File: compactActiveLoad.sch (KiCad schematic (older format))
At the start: 35 parts, among them CON1 Keystone_3002, CON2 Keystone_3002, CON3 LOAD, CON4 +12V, CON5 MOD, CON6 FAN, P1 1k, Q1 IRLR024NPBF, Q2 IRLR024NPBF, SW1 Bat/Ext, SW2 Ext/Int, U1 LMV116MF, U2 LP2981A-50DBVR

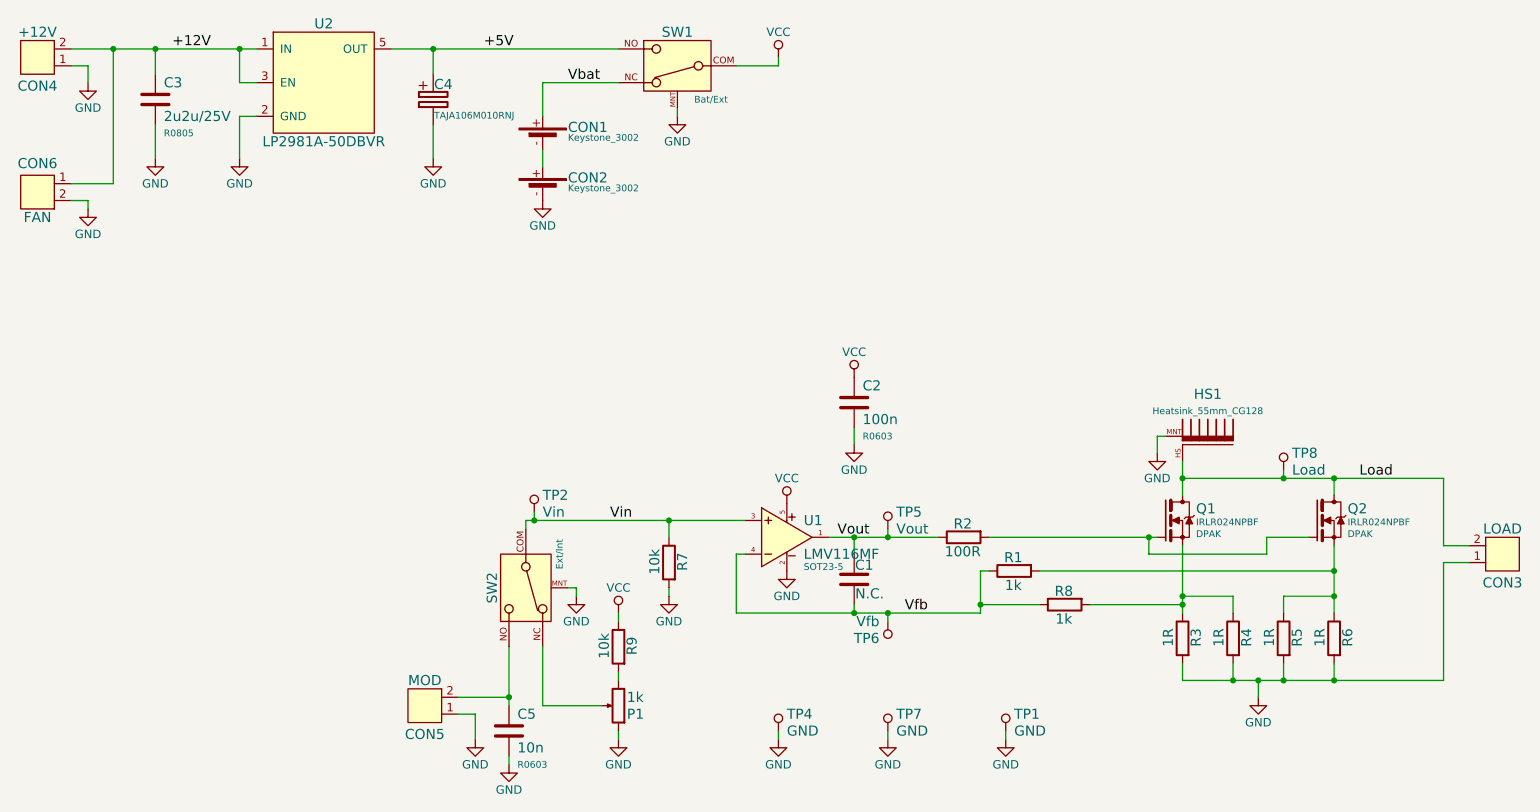
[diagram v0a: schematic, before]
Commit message: Some changes
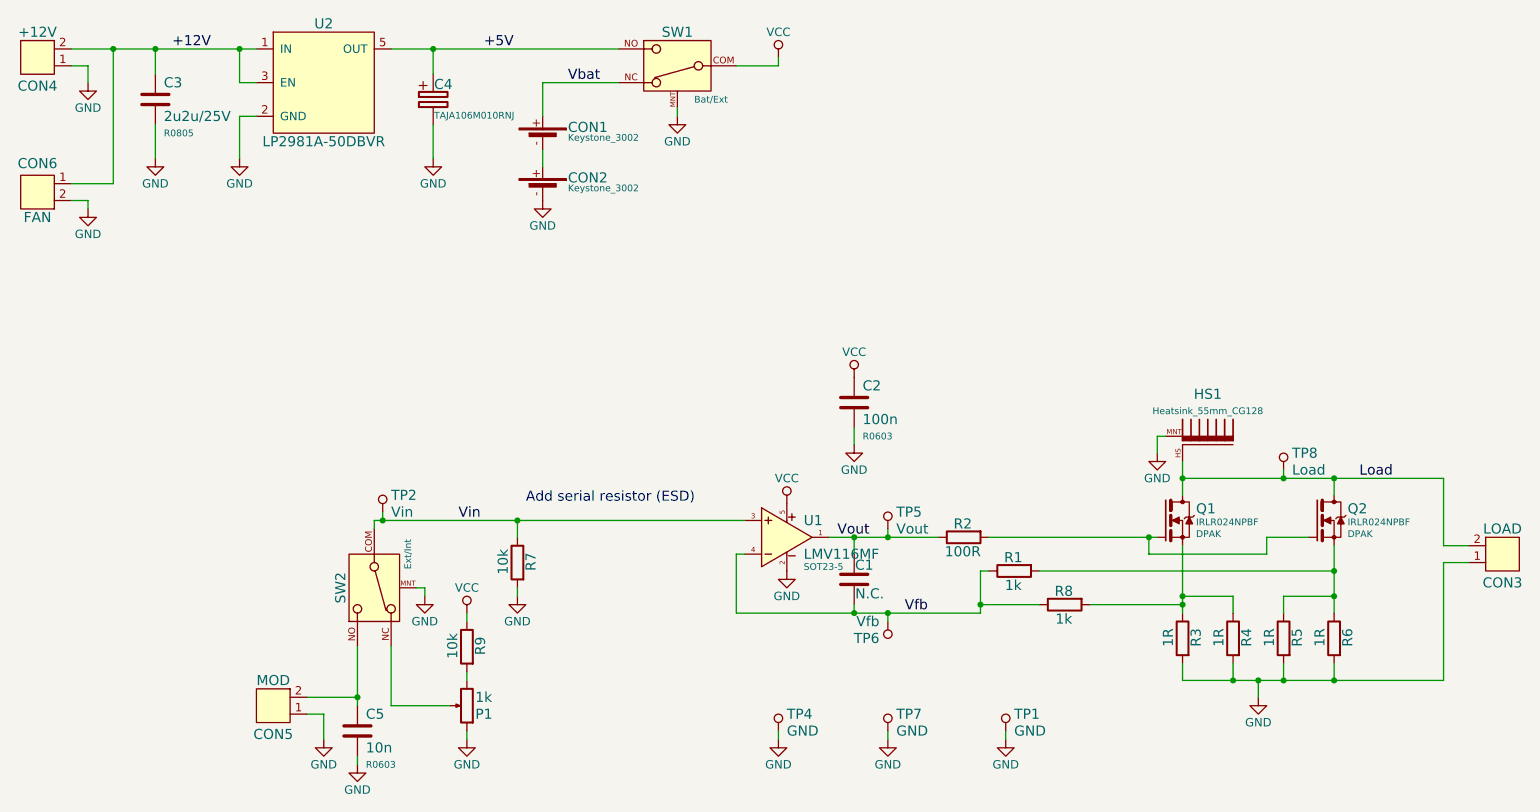
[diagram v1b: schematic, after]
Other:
- note added: "Add serial resistor (ESD)"
- moved on the sheet: C5, CON5, P1, R7, R9, SW2, TP2
